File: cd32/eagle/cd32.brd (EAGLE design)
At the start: 128.2 x 35.2 mm, 2 parts, among them CN1 CD32-EXPANSION, CN2 CD32-EXPANSION

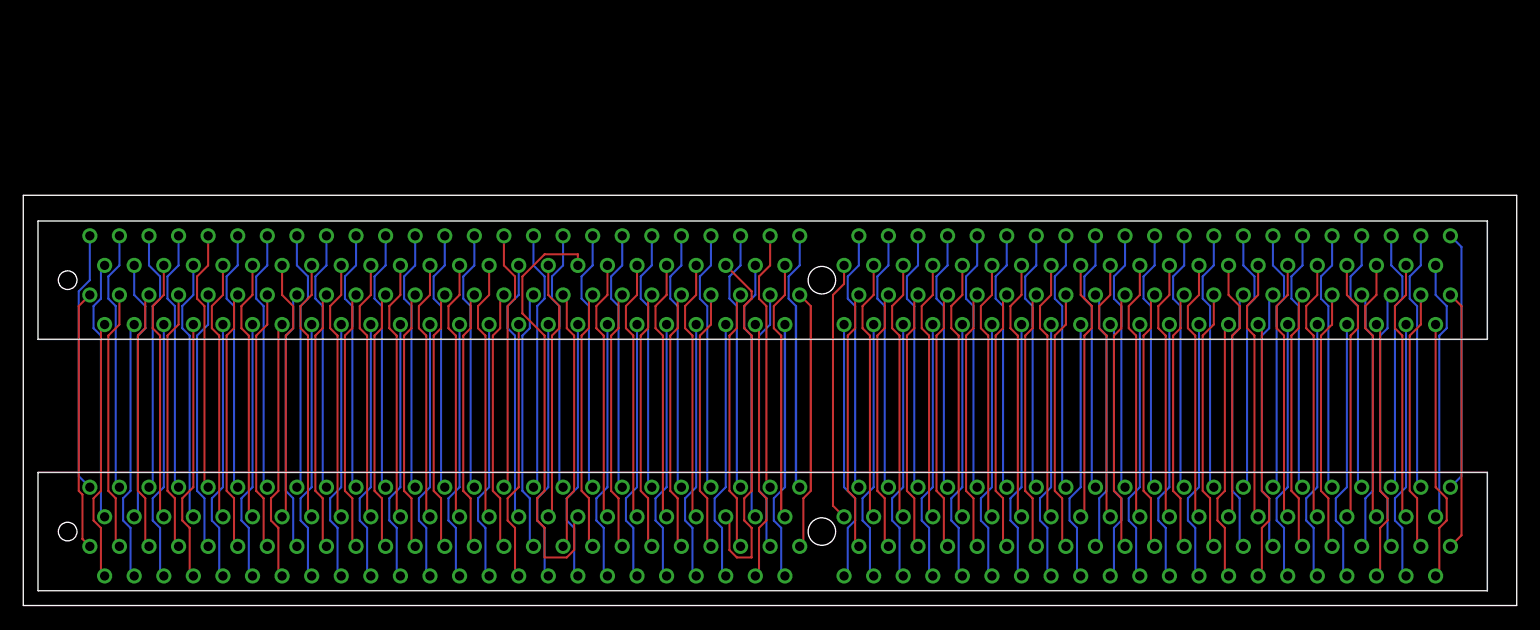
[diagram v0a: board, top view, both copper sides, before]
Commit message: updates.. adjusted board shape... not finished yet Added Maxim RS232 chip
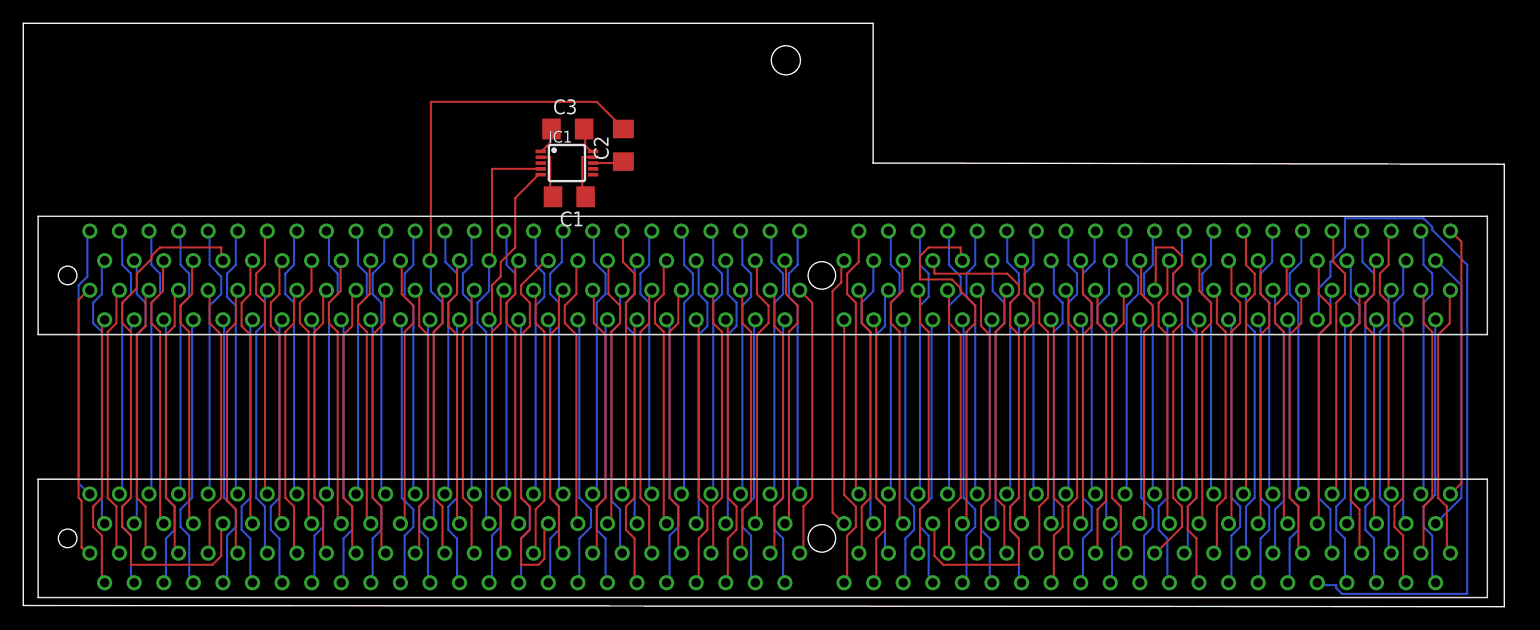
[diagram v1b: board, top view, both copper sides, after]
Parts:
- added C1, C2, C3: (no value), eagle-ltspice:C1206
- added IC1: MAX3311, maxim:UMAX10
- moved CN1 0.58 mm to (63.5, 5.77)
- moved CN2 0.41 mm to (63.5, 28.3)
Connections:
- new net GND: C3.2, IC1.10
- new net N$1: C1.1, IC1.9
- new net N$2: C1.2, IC1.2
- new net N$3: C2.1, IC1.8
- new net VCC: C3.1, IC1.1
- net +12V@1: now also C2.2
- net _RXD: now also IC1.5
- net _TXD: now also IC1.4
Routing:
- net GND@2: track 22.4 -> 63.7 mm
- net +12V@1: track 22.4 -> 54.6 mm
- net AR: track 22.4 -> 46.9 mm
- net D6: track 22.4 -> 44.6 mm
- net _RXD: track 22.4 -> 38.0 mm
- net NC@11: track 37.7 -> 23.5 mm
- net _TXD: track 22.4 -> 35.6 mm
- net D31: track 22.4 -> 34.0 mm
- net _INT6: track 22.4 -> 34.0 mm
- net D8: track 22.4 -> 32.0 mm
- net _AVEC: track 32.2 -> 23.4 mm
- net N$1: track 0.00 -> 4.44 mm
- net N$2: track 0.00 -> 4.35 mm
- net N$3: track 0.00 -> 2.69 mm
- net GND: track 0.00 -> 2.33 mm
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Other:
- board size 128.2 x 35.2 mm -> 127.2 x 50.1 mm
- board text added: "Terrible Fire CD32 Adaptor (C) 2017 S.J Leary Publushed Under the GNU GPLv2"
